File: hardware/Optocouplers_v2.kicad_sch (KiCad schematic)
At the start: 7 parts

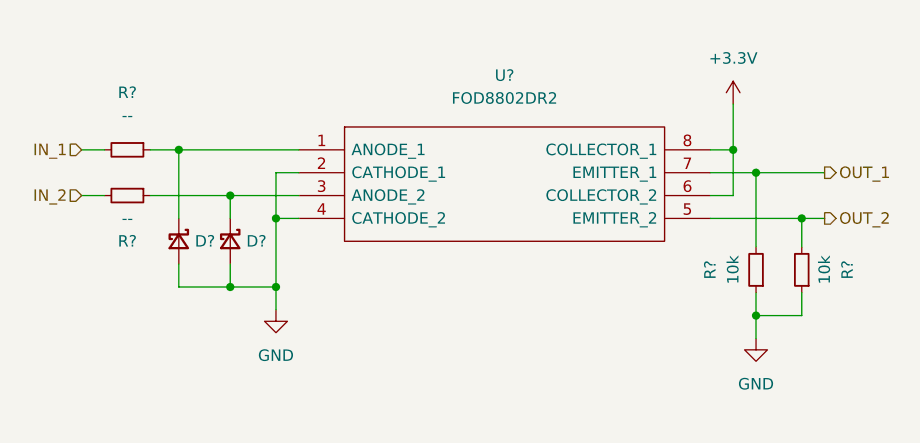
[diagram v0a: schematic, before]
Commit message: changed some footprints for clarity, and made some progress on board
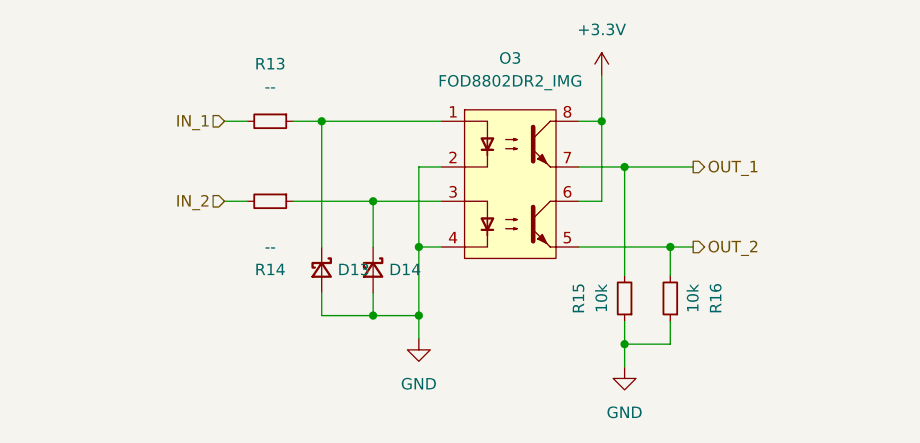
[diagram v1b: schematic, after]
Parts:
- removed U?: FOD8802DR2, SOIC127P600X175-8N, symbol FOD8802DR2:FOD8802DR2
- added O3: FOD8802DR2_IMG, FOD8802DR2:SOIC127P600X175-8N, symbol FOD8802DR2:FOD8802DR2_IMG
- gave numbers to parts that had none: 6
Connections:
- net +3V3: now also O3.6, O3.8
- net GND: now also O3.2, O3.4
- net OUT_1: now also O3.7
- net OUT_2: now also O3.5
- net at D13.1 (K), R13.1: now also O3.1
- net at D14.1 (K), R14.1: now also O3.3
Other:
- moved on the sheet: D13, D14, R13, R14, R15, R16
